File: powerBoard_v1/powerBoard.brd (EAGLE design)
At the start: 81.3 x 58.1 mm, 43 parts, among them IC1 7805T, IC2 317T, IC3 317T, IC4 317T, IC5 7808T, J1 DCJ0202

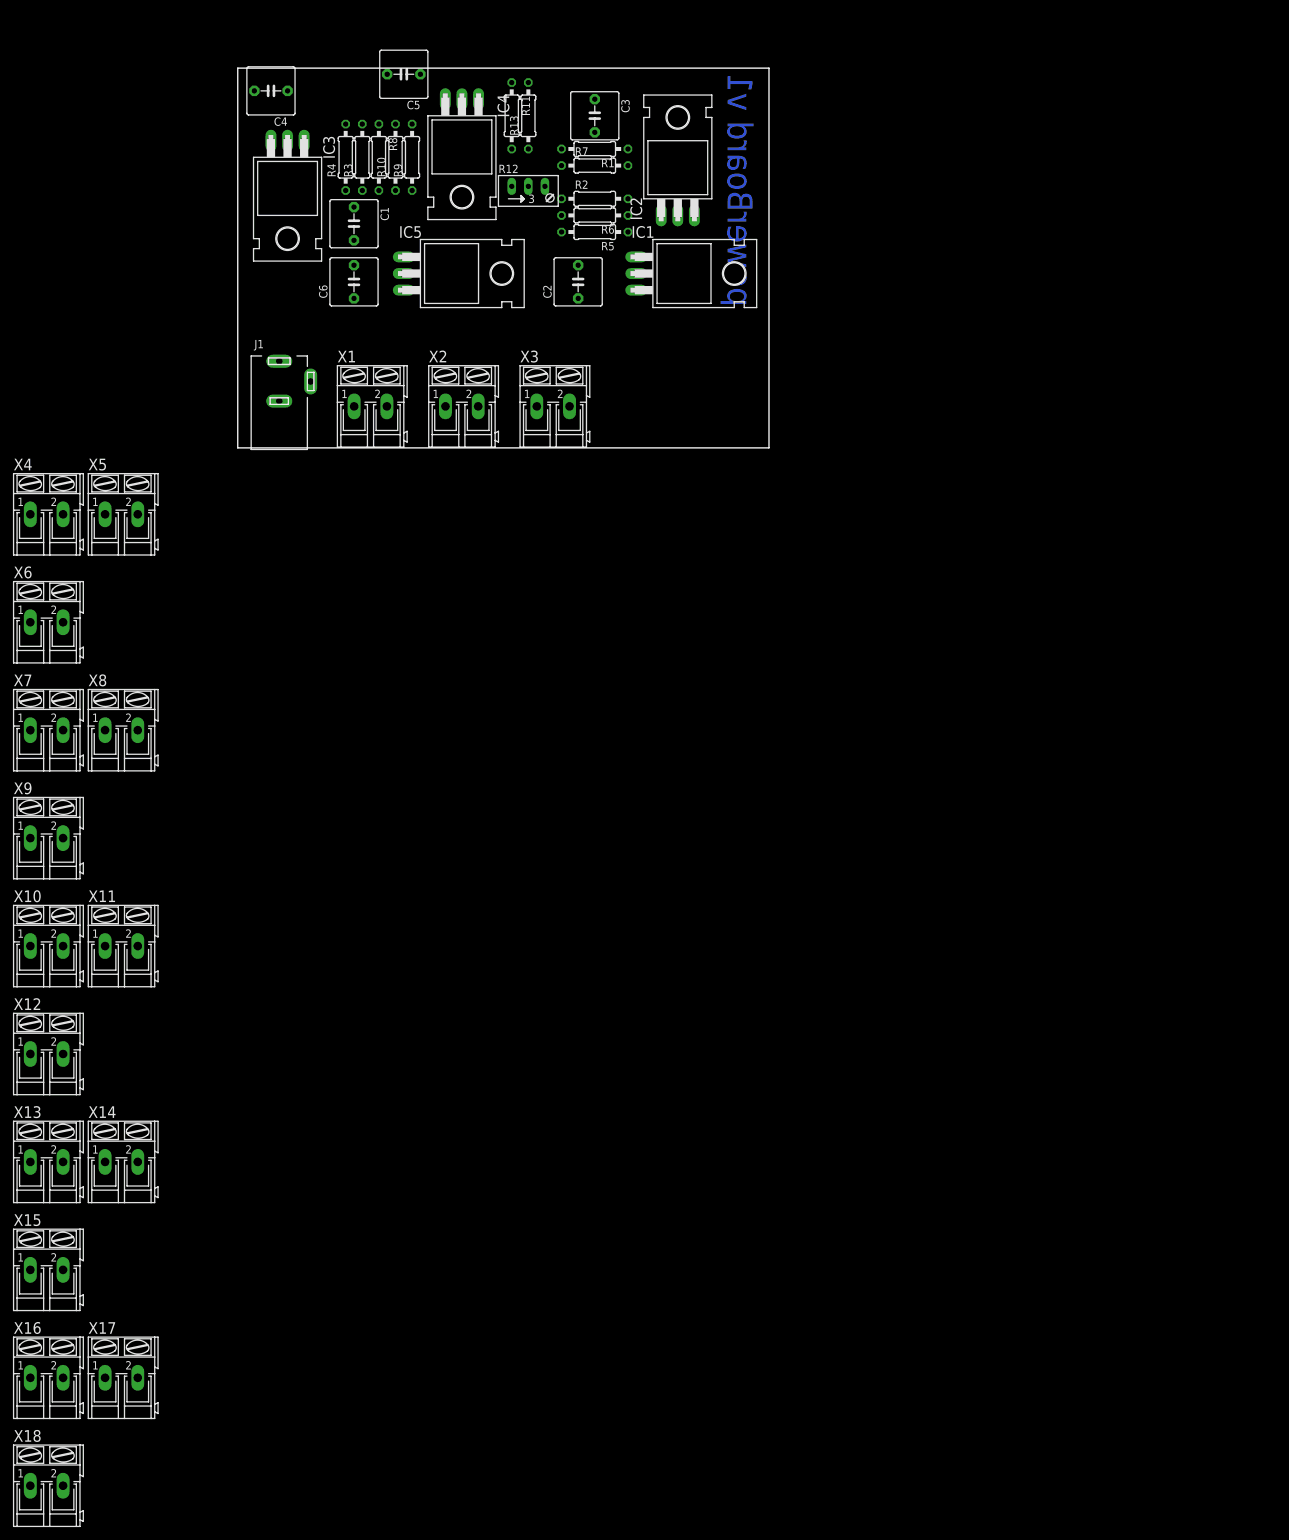
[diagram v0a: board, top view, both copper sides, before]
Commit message: board completed
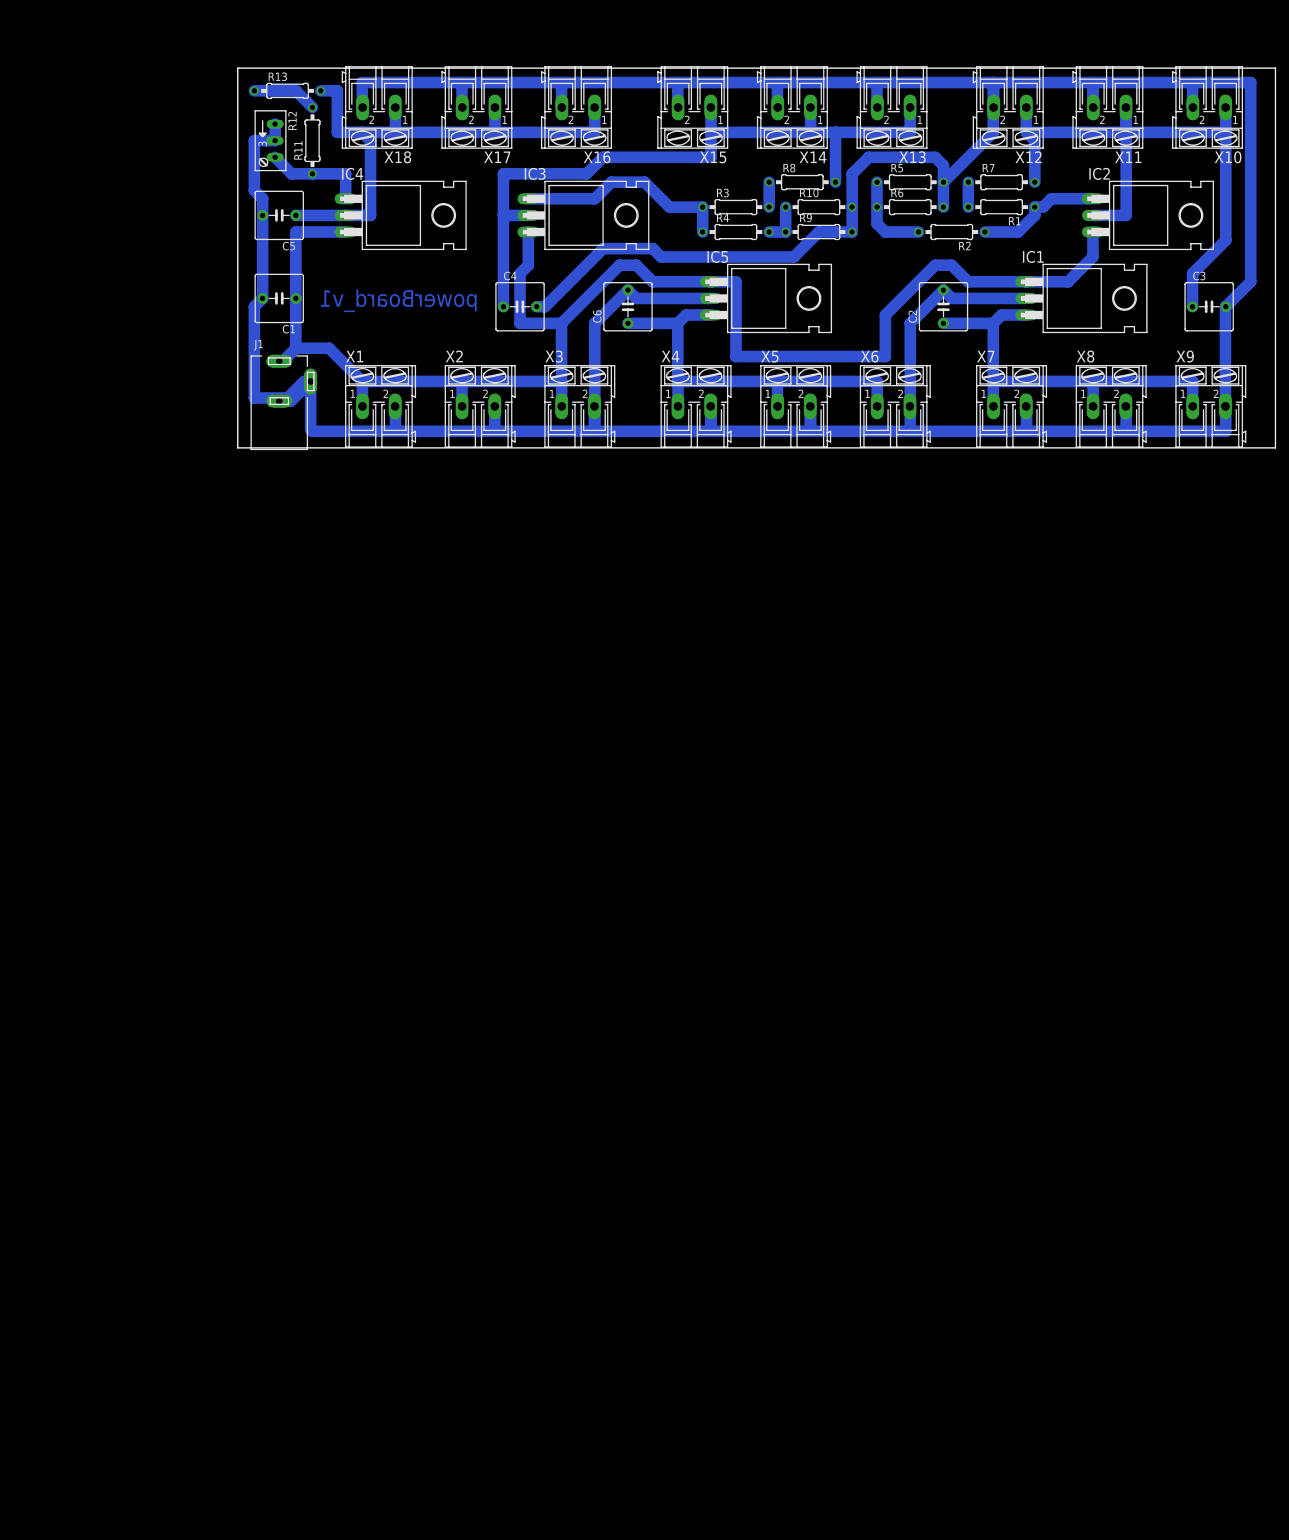
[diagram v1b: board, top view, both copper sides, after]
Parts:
- moved X10 219.2 mm to (148.6, 52.1), turned to 180 degrees
- moved X18 216.9 mm to (21.6, 52.1), turned to 180 degrees
- moved X16 210.6 mm to (52.1, 52.1), turned to 180 degrees
- moved X13 206.9 mm to (100.3, 52.1), turned to 180 degrees
- moved X12 206.6 mm to (118.1, 52.1), turned to 180 degrees
- moved X15 203.5 mm to (69.8, 52.1), turned to 180 degrees
- moved X17 201.8 mm to (36.8, 52.1), turned to 180 degrees
- moved X11 198.2 mm to (133.3, 52.1), turned to 180 degrees
- moved X14 191.3 mm to (85.1, 52.1), turned to 180 degrees
- moved X9 189.7 mm to (148.6, 6.35)
- moved X8 159.0 mm to (133.3, 6.35)
- moved X7 155.4 mm to (118.1, 6.35)
- moved X6 133.7 mm to (100.3, 6.35)
- moved X5 104.2 mm to (85.1, 6.35)
- moved X4 100.4 mm to (69.8, 6.35)
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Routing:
- net GND: track 0.00 -> 650.6 mm
- net +12V: track 0.00 -> 226.1 mm
- net VCC: track 0.00 -> 110.3 mm
- net +3V3: track 0.00 -> 100.5 mm
- net VCC/2: track 0.00 -> 84.4 mm
- net VDD: track 0.00 -> 64.1 mm
- net +5V: track 0.00 -> 64.1 mm
- net N$4: track 0.00 -> 33.1 mm
- net N$2: track 0.00 -> 19.4 mm
- net N$12: track 0.00 -> 15.7 mm
- net N$5: track 0.00 -> 13.2 mm
- net N$13: track 0.00 -> 9.94 mm
- net N$9: track 0.00 -> 6.35 mm
- net N$7: track 0.00 -> 3.81 mm
- net N$6: track 0.00 -> 3.81 mm
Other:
- board size 81.3 x 58.1 mm -> 158.7 x 58.1 mm
- board text added: "powerBoard_v1"
- board text removed: "powerBoard v1"
